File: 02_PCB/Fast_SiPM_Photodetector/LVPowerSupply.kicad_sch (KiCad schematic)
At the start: 9 parts, among them IC2 LMR51606XDBVR

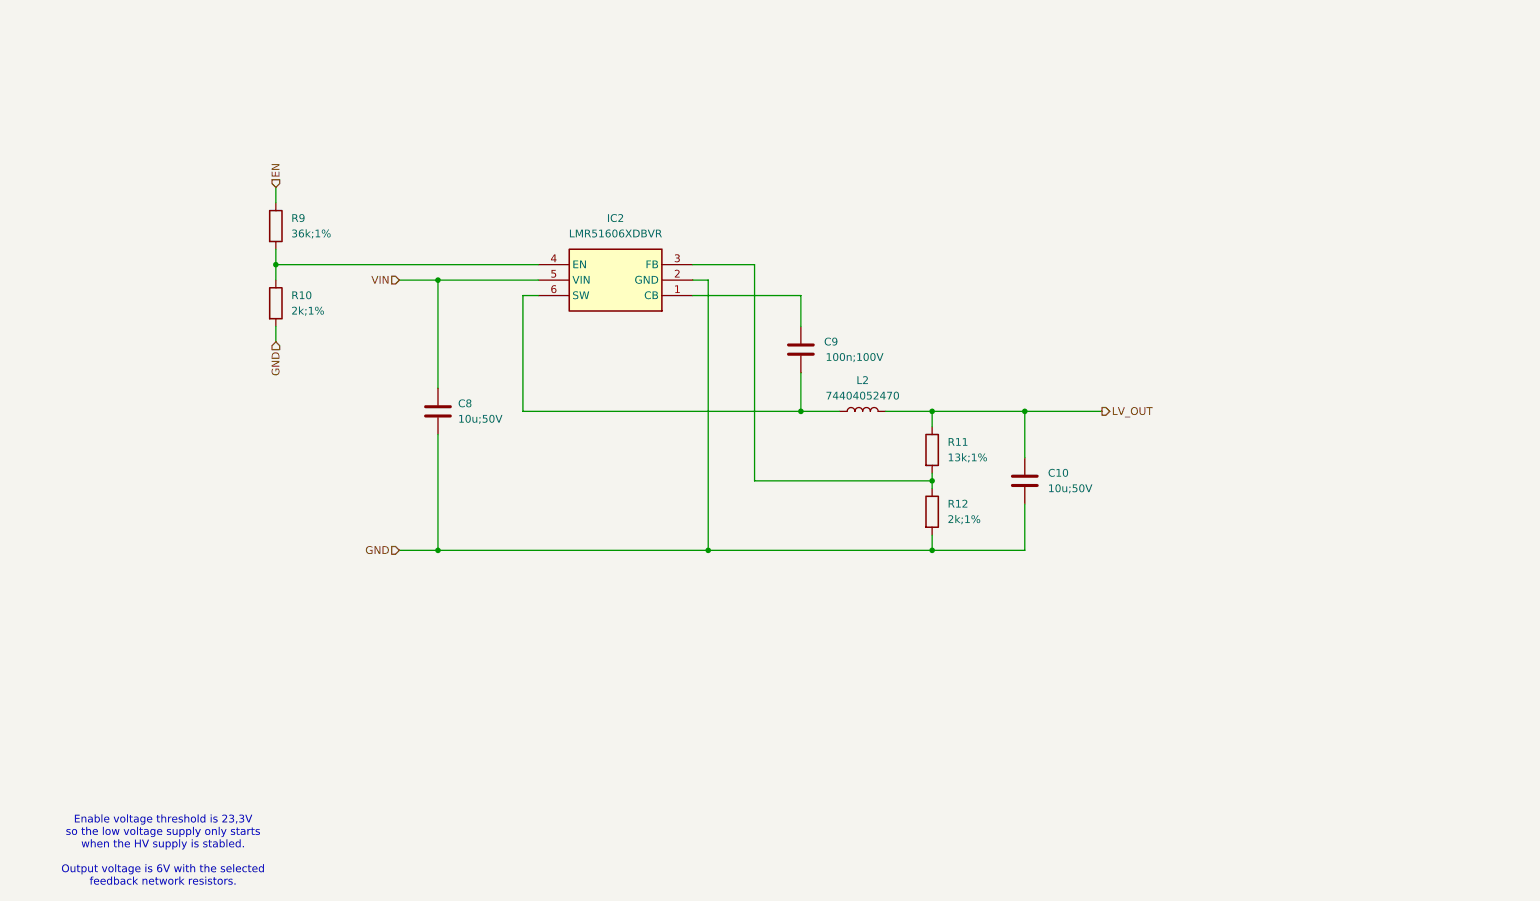
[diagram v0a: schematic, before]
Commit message: feat(detector): update schematic and pcb after first prototype
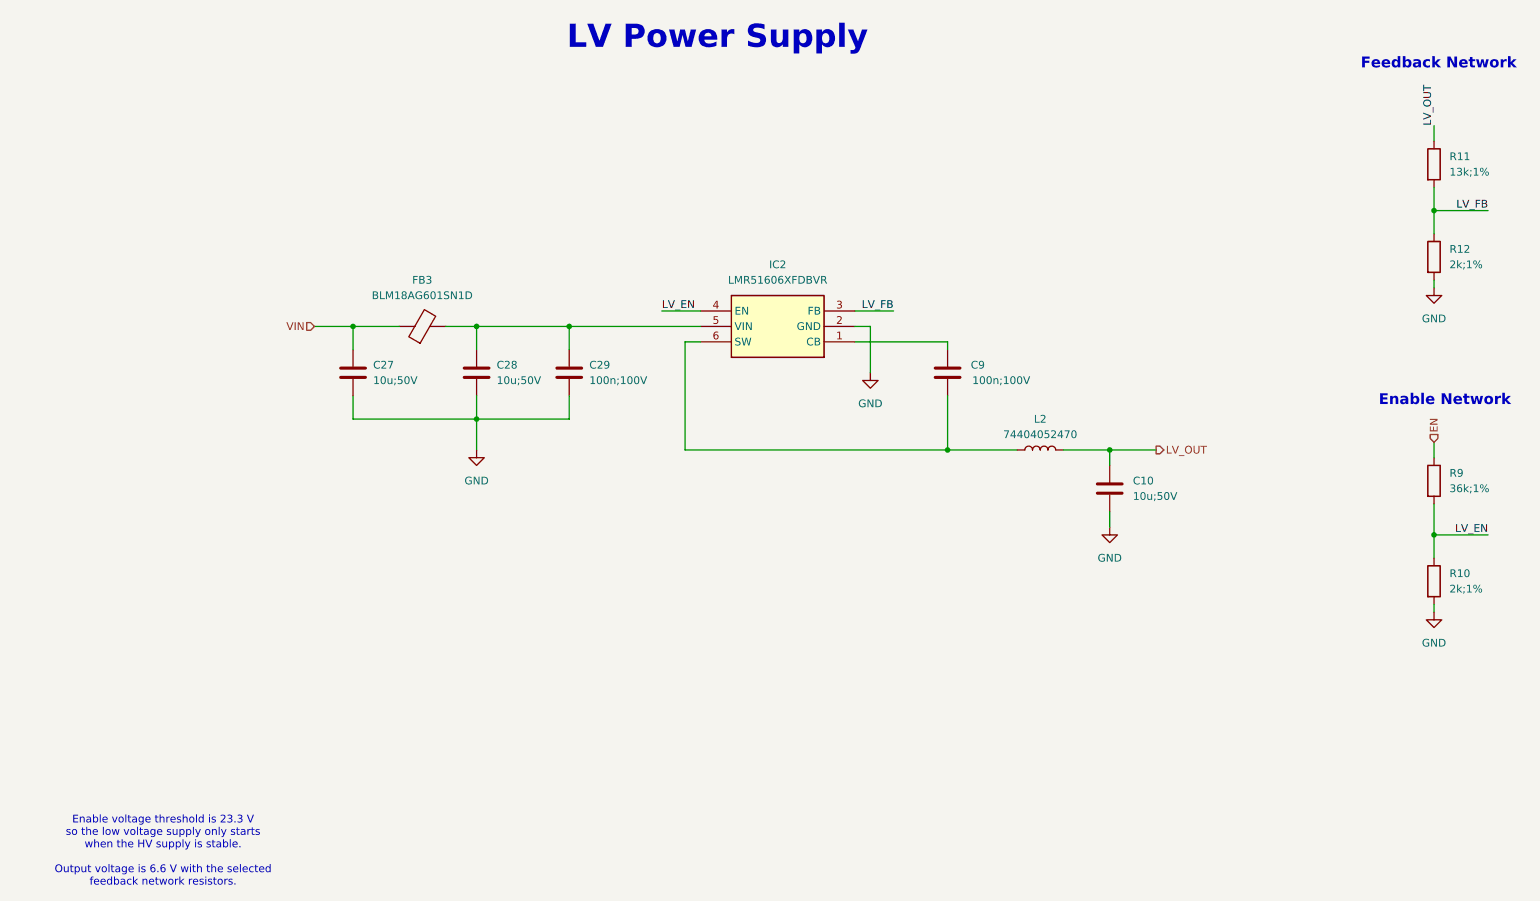
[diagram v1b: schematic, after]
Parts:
- removed C8: 10u;50V, Capacitor_SMD:C_1206_3216Metric, symbol Device:C
- added C27, C28: 10u;50V, Capacitor_SMD:C_1206_3216Metric, symbol Device:C
- added C29: 100n;100V, Capacitor_SMD:C_0603_1608Metric, symbol Device:C
- added FB3: BLM18AG601SN1D, Inductor_SMD:L_0603_1608Metric, symbol Device:FerriteBead
- IC2: value LMR51606XDBVR -> LMR51606XFDBVR
- L2: footprint Inductor_SMD:L_Wuerth_MAPI-5020 -> CustomParts:L_Wuerth_MAPI-5020-Custom
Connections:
- net GND: now also C27.1, C28.1, C29.1
- net VIN: now also C27.2, FB3.1; no longer IC2.5 (VIN)
- net LV_FB: now reaches IC2.3 (FB), R11.2, R12.1
- net LV_EN: now reaches IC2.4 (EN), R10.1, R9.2
- new net: C28.2, C29.2, FB3.2, IC2.5 (VIN)
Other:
- note added: "Enable Network"
- note added: "Enable voltage threshold is 23.3 V so the low voltage supply only starts when the HV supply is stable. Output voltage is 6.6 V with the selected feedback network resistors."
- note added: "Feedback Network"
- note added: "LV Power Supply"
- note removed: "Enable voltage threshold is 23,3V so the low voltage supply only starts when the HV supply is stabled. Output voltage is 6V with the selected feedback network resistors."
- moved on the sheet: C10, C9, IC2, L2, R11, R12
